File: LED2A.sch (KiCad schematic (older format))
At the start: 16 parts

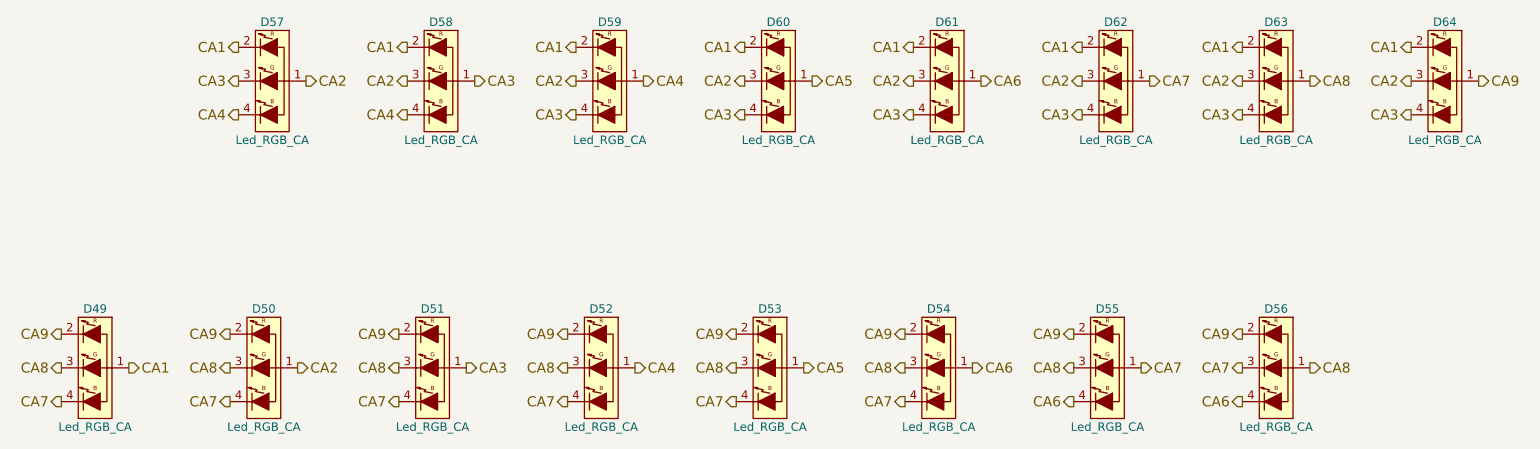
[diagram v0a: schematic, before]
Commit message: Did some visual cleanup.
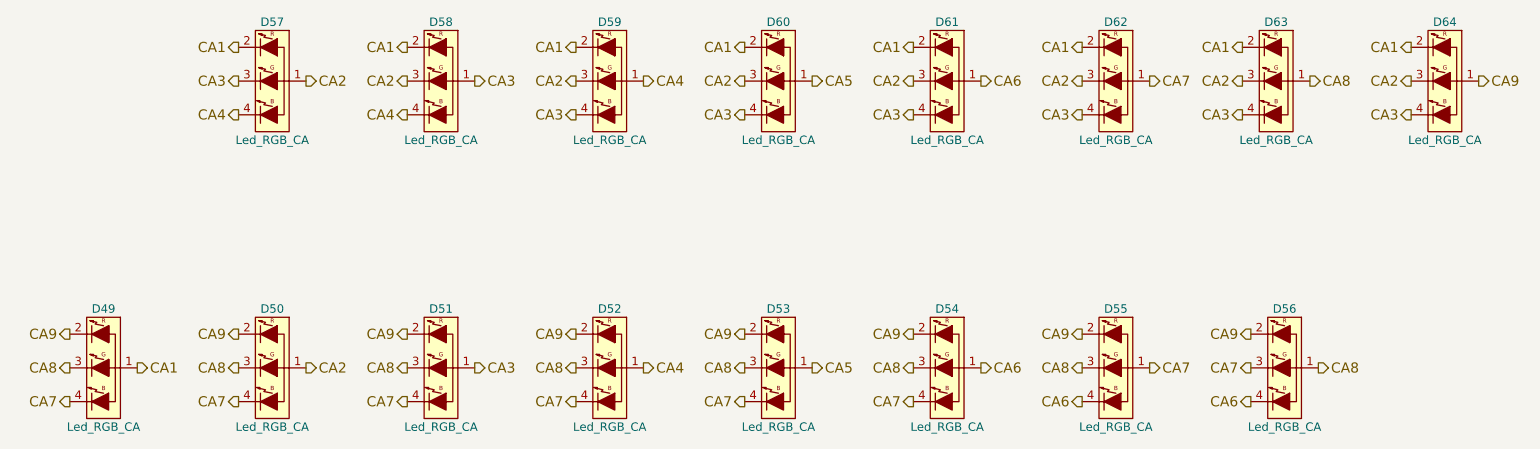
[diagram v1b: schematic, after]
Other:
- moved on the sheet: D49, D50, D51, D52, D53, D54, D55, D56
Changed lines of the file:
@@
 $Descr A4 11693 8268
 encoding utf-8
-Sheet 5 6
+Sheet 3 6
 Title ""
 Date ""
@@
 Text HLabel 9750 1550 0    60   Output ~ 0
 CA1
-Text HLabel 2150 3450 2    60   Output ~ 0
-CA1
-Text HLabel 1750 3650 0    60   Output ~ 0
-CA7
-Text HLabel 1750 3450 0    60   Output ~ 0
-CA8
-Text HLabel 1750 3250 0    60   Output ~ 0
-CA9
-Text HLabel 2750 3650 0    60   Output ~ 0
-CA7
-Text HLabel 2750 3450 0    60   Output ~ 0
-CA8
-Text HLabel 2750 3250 0    60   Output ~ 0
-CA9
-Text HLabel 3150 3450 2    60   Output ~ 0
-CA2
-Text HLabel 3750 3650 0    60   Output ~ 0
-CA7
-Text HLabel 3750 3450 0    60   Output ~ 0
-CA8
-Text HLabel 3750 3250 0    60   Output ~ 0
-CA9
-Text HLabel 4150 3450 2    60   Output ~ 0
-CA3
-Text HLabel 4750 3650 0    60   Output ~ 0
-CA7
-Text HLabel 4750 3450 0    60   Output ~ 0
-CA8
-Text HLabel 4750 3250 0    60   Output ~ 0
-CA9
-Text HLabel 5150 3450 2    60   Output ~ 0
+Text HLabel 2200 3450 2    60   Output ~ 0
+CA1
+Text HLabel 1800 3650 0    60   Output ~ 0
+CA7
+Text HLabel 1800 3450 0    60   Output ~ 0
+CA8
+Text HLabel 1800 3250 0    60   Output ~ 0
+CA9
+Text HLabel 2800 3650 0    60   Output ~ 0
+CA7
+Text HLabel 2800 3450 0    60   Output ~ 0
+CA8
+Text HLabel 2800 3250 0    60   Output ~ 0
+CA9
+Text HLabel 3200 3450 2    60   Output ~ 0
+CA2
+Text HLabel 3800 3650 0    60   Output ~ 0
+CA7
+Text HLabel 3800 3450 0    60   Output ~ 0
+CA8
+Text HLabel 3800 3250 0    60   Output ~ 0
+CA9
+Text HLabel 4200 3450 2    60   Output ~ 0
+CA3
+Text HLabel 4800 3650 0    60   Output ~ 0
+CA7
+Text HLabel 4800 3450 0    60   Output ~ 0
+CA8
+Text HLabel 4800 3250 0    60   Output ~ 0
+CA9
+Text HLabel 5200 3450 2    60   Output ~ 0
 CA4
-Text HLabel 5750 3650 0    60   Output ~ 0
-CA7
-Text HLabel 5750 3450 0    60   Output ~ 0
-CA8
-Text HLabel 5750 3250 0    60   Output ~ 0
-CA9
-Text HLabel 6150 3450 2    60   Output ~ 0
+Text HLabel 5800 3650 0    60   Output ~ 0
+CA7
+Text HLabel 5800 3450 0    60   Output ~ 0
+CA8
+Text HLabel 5800 3250 0    60   Output ~ 0
+CA9
+Text HLabel 6200 3450 2    60   Output ~ 0
 CA5
-Text HLabel 6750 3650 0    60   Output ~ 0
-CA7
-Text HLabel 6750 3450 0    60   Output ~ 0
-CA8
-Text HLabel 6750 3250 0    60   Output ~ 0
-CA9
-Text HLabel 7150 3450 2    60   Output ~ 0
+Text HLabel 6800 3650 0    60   Output ~ 0
+CA7
+Text HLabel 6800 3450 0    60   Output ~ 0
+CA8
+Text HLabel 6800 3250 0    60   Output ~ 0
+CA9
+Text HLabel 7200 3450 2    60   Output ~ 0
 CA6
-Text HLabel 8150 3450 2    60   Output ~ 0
-CA7
-Text HLabel 7750 3450 0    60   Output ~ 0
-CA8
-Text HLabel 7750 3250 0    60   Output ~ 0
-CA9
-Text HLabel 7750 3650 0    60   Output ~ 0
+Text HLabel 8200 3450 2    60   Output ~ 0
+CA7
+Text HLabel 7800 3450 0    60   Output ~ 0
+CA8
+Text HLabel 7800 3250 0    60   Output ~ 0
+CA9
+Text HLabel 7800 3650 0    60   Output ~ 0
 CA6
-Text HLabel 8750 3250 0    60   Output ~ 0
-CA9
-Text HLabel 9150 3450 2    60   Output ~ 0
-CA8
-Text HLabel 8750 3650 0    60   Output ~ 0
+Text HLabel 8800 3250 0    60   Output ~ 0
+CA9
+Text HLabel 9200 3450 2    60   Output ~ 0
+CA8
+Text HLabel 8800 3650 0    60   Output ~ 0
 CA6
-Text HLabel 8750 3450 0    60   Output ~ 0
+Text HLabel 8800 3450 0    60   Output ~ 0
 CA7
 $Comp
@@
 L Led_RGB_CA D49
 U 1 1 56CE590E
-P 1950 3450
-F 0 "D49" H 1950 3800 50  0000 C CNN
-F 1 "Led_RGB_CA" H 1950 3100 50  0000 C CNN
-F 2 "mx2a:RGB" H 1905 3400 50  0001 C CNN
-F 3 "" H 1905 3400 50  0000 C CNN
-	1    1950 3450
+P 2000 3450
+F 0 "D49" H 2000 3800 50  0000 C CNN
+F 1 "Led_RGB_CA" H 2000 3100 50  0000 C CNN
+F 2 "mx2a:RGB" H 1955 3400 50  0001 C CNN
+F 3 "" H 1955 3400 50  0000 C CNN
+	1    2000 3450
 	1    0    0    -1
 $EndComp
@@
 L Led_RGB_CA D50
 U 1 1 56CE5AD7
-P 2950 3450
-F 0 "D50" H 2950 3800 50  0000 C CNN
-F 1 "Led_RGB_CA" H 2950 3100 50  0000 C CNN
-F 2 "mx2a:RGB" H 2905 3400 50  0001 C CNN
-F 3 "" H 2905 3400 50  0000 C CNN
-	1    2950 3450
+P 3000 3450
+F 0 "D50" H 3000 3800 50  0000 C CNN
+F 1 "Led_RGB_CA" H 3000 3100 50  0000 C CNN
+F 2 "mx2a:RGB" H 2955 3400 50  0001 C CNN
+F 3 "" H 2955 3400 50  0000 C CNN
+	1    3000 3450
 	1    0    0    -1
 $EndComp
@@
 L Led_RGB_CA D51
 U 1 1 56CE5B31
-P 3950 3450
-F 0 "D51" H 3950 3800 50  0000 C CNN
-F 1 "Led_RGB_CA" H 3950 3100 50  0000 C CNN
-F 2 "mx2a:RGB" H 3905 3400 50  0001 C CNN
-F 3 "" H 3905 3400 50  0000 C CNN
-	1    3950 3450
+P 4000 3450
+F 0 "D51" H 4000 3800 50  0000 C CNN
+F 1 "Led_RGB_CA" H 4000 3100 50  0000 C CNN
+F 2 "mx2a:RGB" H 3955 3400 50  0001 C CNN
+F 3 "" H 3955 3400 50  0000 C CNN
+	1    4000 3450
 	1    0    0    -1
 $EndComp
@@
 L Led_RGB_CA D52
 U 1 1 56CE5B86
-P 4950 3450
-F 0 "D52" H 4950 3800 50  0000 C CNN
-F 1 "Led_RGB_CA" H 4950 3100 50  0000 C CNN
-F 2 "mx2a:RGB" H 4905 3400 50  0001 C CNN
-F 3 "" H 4905 3400 50  0000 C CNN
-	1    4950 3450
+P 5000 3450
+F 0 "D52" H 5000 3800 50  0000 C CNN
+F 1 "Led_RGB_CA" H 5000 3100 50  0000 C CNN
+F 2 "mx2a:RGB" H 4955 3400 50  0001 C CNN
+F 3 "" H 4955 3400 50  0000 C CNN
+	1    5000 3450
 	1    0    0    -1
 $EndComp
@@
 L Led_RGB_CA D53
 U 1 1 56CE5D1E
-P 5950 3450
-F 0 "D53" H 5950 3800 50  0000 C CNN
-F 1 "Led_RGB_CA" H 5950 3100 50  0000 C CNN
-F 2 "mx2a:RGB" H 5905 3400 50  0001 C CNN
-F 3 "" H 5905 3400 50  0000 C CNN
-	1    5950 3450
+P 6000 3450
+F 0 "D53" H 6000 3800 50  0000 C CNN
+F 1 "Led_RGB_CA" H 6000 3100 50  0000 C CNN
+F 2 "mx2a:RGB" H 5955 3400 50  0001 C CNN
+F 3 "" H 5955 3400 50  0000 C CNN
+	1    6000 3450
 	1    0    0    -1
 $EndComp
@@
 L Led_RGB_CA D54
 U 1 1 56CE5D71
-P 6950 3450
-F 0 "D54" H 6950 3800 50  0000 C CNN
-F 1 "Led_RGB_CA" H 6950 3100 50  0000 C CNN
-F 2 "mx2a:RGB" H 6905 3400 50  0001 C CNN
-F 3 "" H 6905 3400 50  0000 C CNN
-	1    6950 3450
+P 7000 3450
+F 0 "D54" H 7000 3800 50  0000 C CNN
+F 1 "Led_RGB_CA" H 7000 3100 50  0000 C CNN
+F 2 "mx2a:RGB" H 6955 3400 50  0001 C CNN
+F 3 "" H 6955 3400 50  0000 C CNN
+	1    7000 3450
 	1    0    0    -1
 $EndComp
@@
 L Led_RGB_CA D55
 U 1 1 56CE5EE3
-P 7950 3450
-F 0 "D55" H 7950 3800 50  0000 C CNN
-F 1 "Led_RGB_CA" H 7950 3100 50  0000 C CNN
-F 2 "mx2a:RGB" H 7905 3400 50  0001 C CNN
-F 3 "" H 7905 3400 50  0000 C CNN
-	1    7950 3450
+P 8000 3450
+F 0 "D55" H 8000 3800 50  0000 C CNN
+F 1 "Led_RGB_CA" H 8000 3100 50  0000 C CNN
+F 2 "mx2a:RGB" H 7955 3400 50  0001 C CNN
+F 3 "" H 7955 3400 50  0000 C CNN
+	1    8000 3450
 	1    0    0    -1
 $EndComp
@@
 L Led_RGB_CA D56
 U 1 1 56CE5F40
-P 8950 3450
-F 0 "D56" H 8950 3800 50  0000 C CNN
-F 1 "Led_RGB_CA" H 8950 3100 50  0000 C CNN
-F 2 "mx2a:RGB" H 8905 3400 50  0001 C CNN
-F 3 "" H 8905 3400 50  0000 C CNN
-	1    8950 3450
-	1    0    0    -1
-$EndComp
+P 9000 3450
+F 0 "D56" H 9000 3800 50  0000 C CNN
+F 1 "Led_RGB_CA" H 9000 3100 50  0000 C CNN
+F 2 "mx2a:RGB" H 8955 3400 50  0001 C CNN
+F 3 "" H 8955 3400 50  0000 C CNN
+	1    9000 3450
+	1    0    0    -1
+$EndComp

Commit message: Switched to a different USB Port and 100uF Cap
also added a USB-Debug Header and did some cleanup
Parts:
- D49, D50, D51, D52, D53, D54, D55, D56, D57, D58, D59, D60, D61, D62, D63, D64: footprint mx2a:RGB -> libs.pretty:RGB
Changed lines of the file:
@@
 U 1 1 56CDDA8B
 P 3000 1750
+AR Path="/56CDDA8B" Ref="D57"  Part="1"
+AR Path="/5735BDF5/56CDDA8B" Ref="D57"  Part="1"
 F 0 "D57" H 3000 2100 50  0000 C CNN
 F 1 "Led_RGB_CA" H 3000 1400 50  0000 C CNN
-F 2 "mx2a:RGB" H 2955 1700 50  0001 C CNN
+F 2 "libs.pretty:RGB" H 2955 1700 50  0001 C CNN
 F 3 "" H 2955 1700 50  0000 C CNN
 	1    3000 1750
@@
 U 1 1 56CDDAD5
 P 4000 1750
+AR Path="/56CDDAD5" Ref="D58"  Part="1"
+AR Path="/5735BDF5/56CDDAD5" Ref="D58"  Part="1"
 F 0 "D58" H 4000 2100 50  0000 C CNN
 F 1 "Led_RGB_CA" H 4000 1400 50  0000 C CNN
-F 2 "mx2a:RGB" H 3955 1700 50  0001 C CNN
+F 2 "libs.pretty:RGB" H 3955 1700 50  0001 C CNN
 F 3 "" H 3955 1700 50  0000 C CNN
 	1    4000 1750
@@
 U 1 1 56CDDB75
 P 5000 1750
+AR Path="/56CDDB75" Ref="D59"  Part="1"
+AR Path="/5735BDF5/56CDDB75" Ref="D59"  Part="1"
 F 0 "D59" H 5000 2100 50  0000 C CNN
 F 1 "Led_RGB_CA" H 5000 1400 50  0000 C CNN
-F 2 "mx2a:RGB" H 4955 1700 50  0001 C CNN
+F 2 "libs.pretty:RGB" H 4955 1700 50  0001 C CNN
 F 3 "" H 4955 1700 50  0000 C CNN
 	1    5000 1750
@@
 U 1 1 56CDDC19
 P 6000 1750
+AR Path="/56CDDC19" Ref="D60"  Part="1"
+AR Path="/5735BDF5/56CDDC19" Ref="D60"  Part="1"
 F 0 "D60" H 6000 2100 50  0000 C CNN
 F 1 "Led_RGB_CA" H 6000 1400 50  0000 C CNN
-F 2 "mx2a:RGB" H 5955 1700 50  0001 C CNN
+F 2 "libs.pretty:RGB" H 5955 1700 50  0001 C CNN
 F 3 "" H 5955 1700 50  0000 C CNN
 	1    6000 1750
@@
 U 1 1 56CDDD1F
 P 7000 1750
+AR Path="/56CDDD1F" Ref="D61"  Part="1"
+AR Path="/5735BDF5/56CDDD1F" Ref="D61"  Part="1"
 F 0 "D61" H 7000 2100 50  0000 C CNN
 F 1 "Led_RGB_CA" H 7000 1400 50  0000 C CNN
-F 2 "mx2a:RGB" H 6955 1700 50  0001 C CNN
+F 2 "libs.pretty:RGB" H 6955 1700 50  0001 C CNN
 F 3 "" H 6955 1700 50  0000 C CNN
 	1    7000 1750
@@
 U 1 1 56CDDD5A
 P 8000 1750
+AR Path="/56CDDD5A" Ref="D62"  Part="1"
+AR Path="/5735BDF5/56CDDD5A" Ref="D62"  Part="1"
 F 0 "D62" H 8000 2100 50  0000 C CNN
 F 1 "Led_RGB_CA" H 8000 1400 50  0000 C CNN
-F 2 "mx2a:RGB" H 7955 1700 50  0001 C CNN
+F 2 "libs.pretty:RGB" H 7955 1700 50  0001 C CNN
 F 3 "" H 7955 1700 50  0000 C CNN
 	1    8000 1750
@@
 U 1 1 56CDDE52
 P 8950 1750
+AR Path="/56CDDE52" Ref="D63"  Part="1"
+AR Path="/5735BDF5/56CDDE52" Ref="D63"  Part="1"
 F 0 "D63" H 8950 2100 50  0000 C CNN
 F 1 "Led_RGB_CA" H 8950 1400 50  0000 C CNN
-F 2 "mx2a:RGB" H 8905 1700 50  0001 C CNN
+F 2 "libs.pretty:RGB" H 8905 1700 50  0001 C CNN
 F 3 "" H 8905 1700 50  0000 C CNN
 	1    8950 1750
@@
 U 1 1 56CDDF9D
 P 9950 1750
+AR Path="/56CDDF9D" Ref="D64"  Part="1"
+AR Path="/5735BDF5/56CDDF9D" Ref="D64"  Part="1"
 F 0 "D64" H 9950 2100 50  0000 C CNN
 F 1 "Led_RGB_CA" H 9950 1400 50  0000 C CNN
-F 2 "mx2a:RGB" H 9905 1700 50  0001 C CNN
+F 2 "libs.pretty:RGB" H 9905 1700 50  0001 C CNN
 F 3 "" H 9905 1700 50  0000 C CNN
 	1    9950 1750
@@
 U 1 1 56CE590E
 P 2000 3450
+AR Path="/56CE590E" Ref="D49"  Part="1"
+AR Path="/5735BDF5/56CE590E" Ref="D49"  Part="1"
 F 0 "D49" H 2000 3800 50  0000 C CNN
 F 1 "Led_RGB_CA" H 2000 3100 50  0000 C CNN
-F 2 "mx2a:RGB" H 1955 3400 50  0001 C CNN
+F 2 "libs.pretty:RGB" H 1955 3400 50  0001 C CNN
 F 3 "" H 1955 3400 50  0000 C CNN
 	1    2000 3450
@@
 U 1 1 56CE5AD7
 P 3000 3450
+AR Path="/56CE5AD7" Ref="D50"  Part="1"
+AR Path="/5735BDF5/56CE5AD7" Ref="D50"  Part="1"
 F 0 "D50" H 3000 3800 50  0000 C CNN
 F 1 "Led_RGB_CA" H 3000 3100 50  0000 C CNN
-F 2 "mx2a:RGB" H 2955 3400 50  0001 C CNN
+F 2 "libs.pretty:RGB" H 2955 3400 50  0001 C CNN
 F 3 "" H 2955 3400 50  0000 C CNN
 	1    3000 3450
@@
 U 1 1 56CE5B31
 P 4000 3450
+AR Path="/56CE5B31" Ref="D51"  Part="1"
+AR Path="/5735BDF5/56CE5B31" Ref="D51"  Part="1"
 F 0 "D51" H 4000 3800 50  0000 C CNN
 F 1 "Led_RGB_CA" H 4000 3100 50  0000 C CNN
-F 2 "mx2a:RGB" H 3955 3400 50  0001 C CNN
+F 2 "libs.pretty:RGB" H 3955 3400 50  0001 C CNN
 F 3 "" H 3955 3400 50  0000 C CNN
 	1    4000 3450
@@
 U 1 1 56CE5B86
 P 5000 3450
+AR Path="/56CE5B86" Ref="D52"  Part="1"
+AR Path="/5735BDF5/56CE5B86" Ref="D52"  Part="1"
 F 0 "D52" H 5000 3800 50  0000 C CNN
 F 1 "Led_RGB_CA" H 5000 3100 50  0000 C CNN
-F 2 "mx2a:RGB" H 4955 3400 50  0001 C CNN
+F 2 "libs.pretty:RGB" H 4955 3400 50  0001 C CNN
 F 3 "" H 4955 3400 50  0000 C CNN
 	1    5000 3450
@@
 U 1 1 56CE5D1E
 P 6000 3450
+AR Path="/56CE5D1E" Ref="D53"  Part="1"
+AR Path="/5735BDF5/56CE5D1E" Ref="D53"  Part="1"
 F 0 "D53" H 6000 3800 50  0000 C CNN
 F 1 "Led_RGB_CA" H 6000 3100 50  0000 C CNN
-F 2 "mx2a:RGB" H 5955 3400 50  0001 C CNN
+F 2 "libs.pretty:RGB" H 5955 3400 50  0001 C CNN
 F 3 "" H 5955 3400 50  0000 C CNN
 	1    6000 3450
@@
 U 1 1 56CE5D71
 P 7000 3450
+AR Path="/56CE5D71" Ref="D54"  Part="1"
+AR Path="/5735BDF5/56CE5D71" Ref="D54"  Part="1"
 F 0 "D54" H 7000 3800 50  0000 C CNN
 F 1 "Led_RGB_CA" H 7000 3100 50  0000 C CNN
-F 2 "mx2a:RGB" H 6955 3400 50  0001 C CNN
+F 2 "libs.pretty:RGB" H 6955 3400 50  0001 C CNN
 F 3 "" H 6955 3400 50  0000 C CNN
 	1    7000 3450
@@
 U 1 1 56CE5EE3
 P 8000 3450
+AR Path="/56CE5EE3" Ref="D55"  Part="1"
+AR Path="/5735BDF5/56CE5EE3" Ref="D55"  Part="1"
 F 0 "D55" H 8000 3800 50  0000 C CNN
 F 1 "Led_RGB_CA" H 8000 3100 50  0000 C CNN
-F 2 "mx2a:RGB" H 7955 3400 50  0001 C CNN
+F 2 "libs.pretty:RGB" H 7955 3400 50  0001 C CNN
 F 3 "" H 7955 3400 50  0000 C CNN
 	1    8000 3450
@@
 U 1 1 56CE5F40
 P 9000 3450
+AR Path="/56CE5F40" Ref="D56"  Part="1"
+AR Path="/5735BDF5/56CE5F40" Ref="D56"  Part="1"
 F 0 "D56" H 9000 3800 50  0000 C CNN
 F 1 "Led_RGB_CA" H 9000 3100 50  0000 C CNN
-F 2 "mx2a:RGB" H 8955 3400 50  0001 C CNN
+F 2 "libs.pretty:RGB" H 8955 3400 50  0001 C CNN
 F 3 "" H 8955 3400 50  0000 C CNN
 	1    9000 3450
